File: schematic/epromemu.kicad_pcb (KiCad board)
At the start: 2 copper layers, 81 x 53.6 mm, 12 parts, among them J1 EPROM Connector, U1 Teensy4.1, U2 74HC245, U3 74HC245, U4 74HC245, U5 74HC245, U6 74LS32

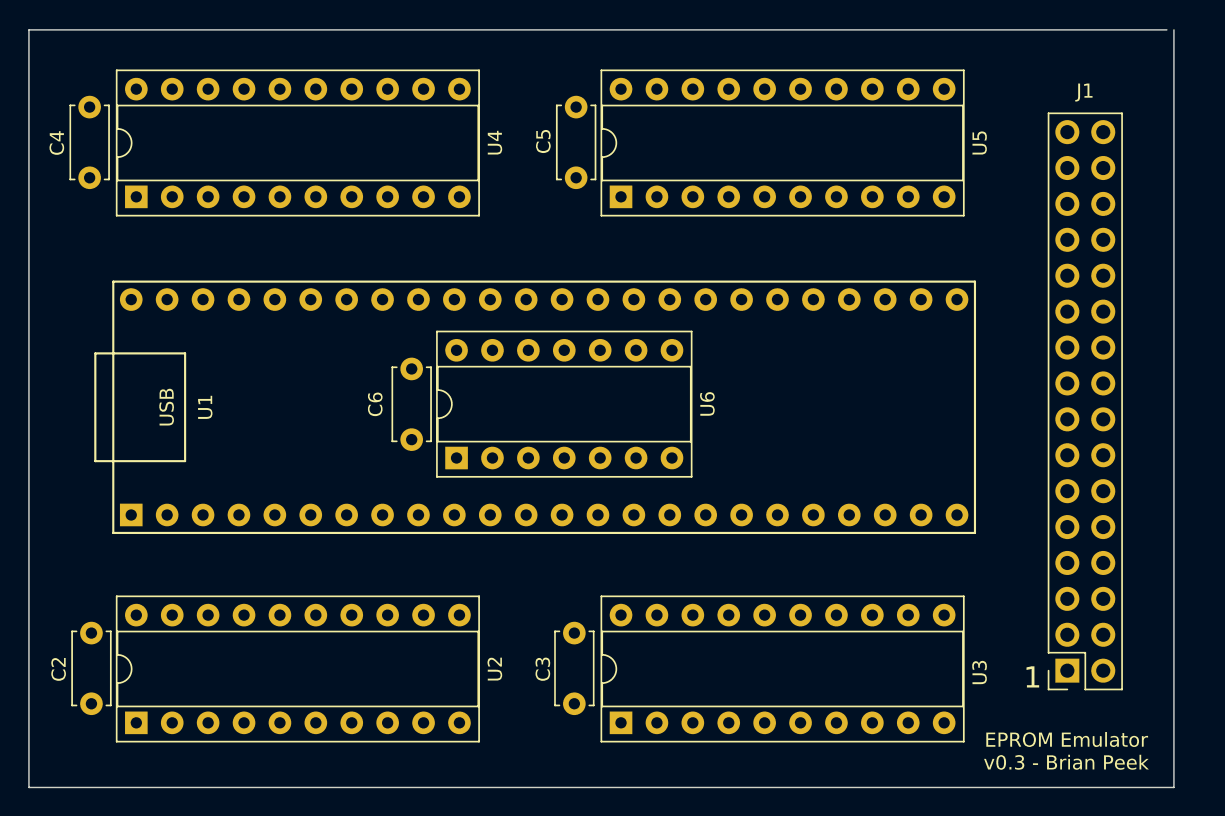
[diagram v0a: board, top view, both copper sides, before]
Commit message: a complete v3?
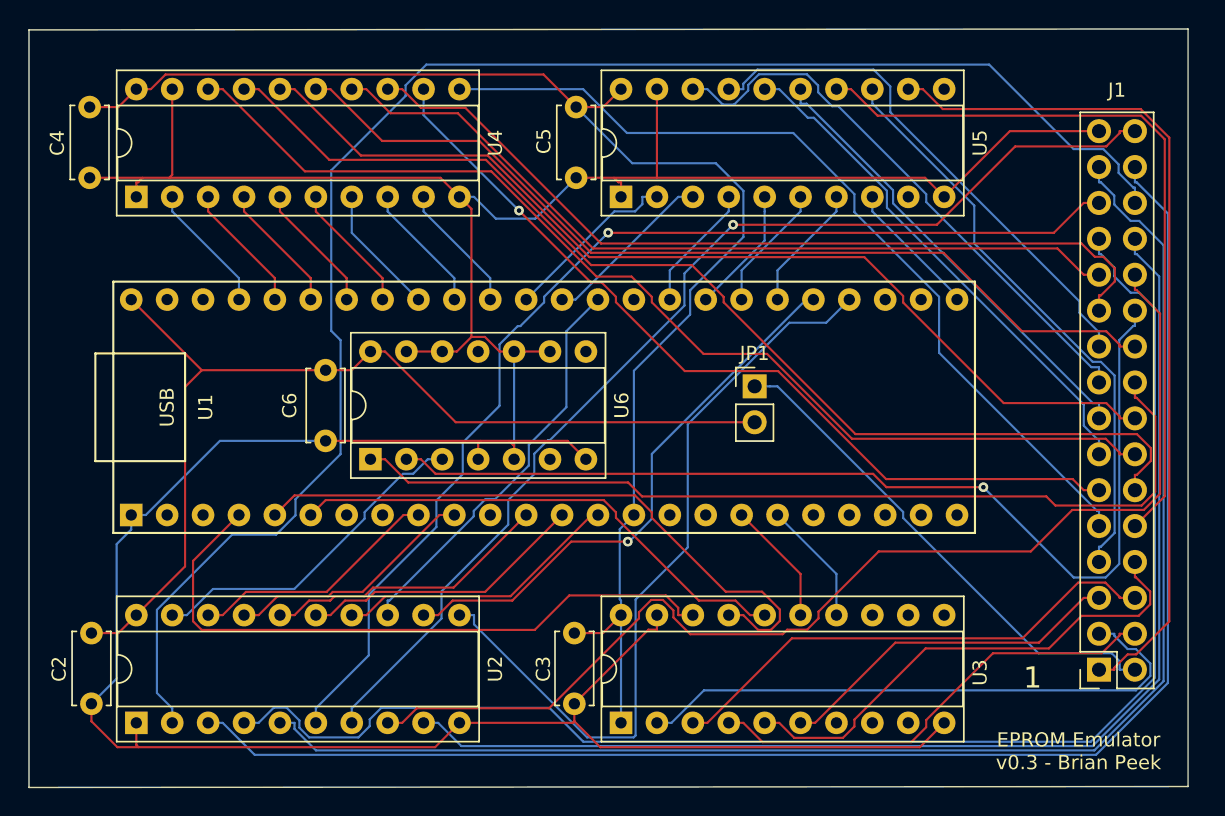
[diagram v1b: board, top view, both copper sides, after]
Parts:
- added JP1: PWR, Connector_PinHeader_2.54mm:PinHeader_1x02_P2.54mm_Vertical, F.Cu at (156.3, 95.9)
- U6: value 74LS32 -> 74HC32
- moved U6 6.09 mm to (129.2, 101.0)
- moved C6 6.09 mm to (126.0, 94.7)
- moved J1 2.24 mm to (183.2, 115.9)
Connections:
- J1 pad 32: +5V -> Net-(J1-Pin_32)
- U1 pad 16: A16_3V3 -> unconnected-(U1-24_A10_TX6_SCL2-Pad16)
- U1 pad 17: A17_3V3 -> unconnected-(U1-25_A11_RX6_SDA2-Pad17)
- U1 pad 2: A19_3V3 -> unconnected-(U1-0_RX1_CRX2_CS1-Pad2)
- U1 pad 25: unconnected-(U1-Pad25) -> A19_3V3
- U1 pad 3: A18_3V3 -> unconnected-(U1-1_TX1_CTX2_MISO1-Pad3)
- U1 pad 4: unconnected-(U1-Pad4) -> A16_3V3
- U1 pad 5: unconnected-(U1-Pad5) -> A17_3V3
- U1 pad 6: unconnected-(U1-Pad6) -> A18_3V3
- U3 pad 13: A15_3V3 -> unconnected-(U3-B5-Pad13)
- U3 pad 14: A14_3V3 -> A15_3V3
- U3 pad 15: A17_3V3 -> A14_3V3
- U3 pad 16: A16_3V3 -> A18_3V3
- U3 pad 17: A18_3V3 -> A17_3V3
- U3 pad 18: A19_3V3 -> A16_3V3
- U3 pad 2: A19_5V -> A16_5V
- U3 pad 3: A18_5V -> A17_5V
- U3 pad 4: A16_5V -> A18_5V
- U3 pad 5: A17_5V -> A14_5V
- U3 pad 6: A14_5V -> A15_5V
- U3 pad 7: A15_5V -> unconnected-(U3-A5-Pad7)
- U5 pad 12: unconnected-(U5-Pad12) -> A19_5V
- U5 pad 8: unconnected-(U5-Pad8) -> A19_3V3
- U6 pad 11: GND -> unconnected-(U6-Pad11)
- U6 pad 6: GND -> unconnected-(U6-Pad6)
- U6 pad 8: GND -> unconnected-(U6-Pad8)
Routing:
- net GND: track 0.00 -> 250.0 mm
- net D5_5V: track 0.00 -> 112.5 mm
- net D4_5V: track 0.00 -> 108.5 mm
- net D2_5V: track 0.00 -> 104.3 mm
- net D0_5V: track 0.00 -> 103.2 mm
- net +3V3: track 0.00 -> 99.4 mm
- net D6_5V: track 0.00 -> 86.6 mm
- net D7_5V: track 0.00 -> 80.5 mm
- net D1_5V: track 0.00 -> 79.0 mm, vias 0 -> 1
- net A8_5V: track 0.00 -> 78.4 mm
- net D3_5V: track 0.00 -> 77.7 mm, vias 0 -> 1
- net A9_5V: track 0.00 -> 76.6 mm
- net CE_5V: track 0.00 -> 72.7 mm, vias 0 -> 1
- net +5V: track 0.00 -> 71.7 mm
- net A11_5V: track 0.00 -> 70.5 mm
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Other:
- board size 81 x 53.6 mm -> 82 x 53.7 mm
